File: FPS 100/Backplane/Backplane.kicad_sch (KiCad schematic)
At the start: 13 parts, among them J2 Conn_02x50_100pin

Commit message: 2026/1/3
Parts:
- added 4408_P3_J1, 4408_P3_J2, 4422_P1_J3, 4422_P1_J4, 4423_P2_J1, 4423_P2_J2, Spare1_J1, Spare1_J2: Conn_02x60_120pin, symbol User:Conn_02x60_120pin
- added 4421_PDP_IF_J1, 4421_PDP_IF_J2, 4429_FMT_J1, 4429_FMT_J2, Spare2_J2, Spare2_J3, Spare2_J4: Conn_02x50_100pin, symbol User:Conn_02x50_100pin
- renumbered J2 to Spare2_J1
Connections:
- net +5V: now also Spare2_J1.1, Spare2_J1.100, Spare2_J1.2, Spare2_J1.99, 4408_P3_J1.1, 4408_P3_J1.119, 4408_P3_J1.120, 4408_P3_J1.2, 4408_P3_J2.1, 4408_P3_J2.119, 4408_P3_J2.120, 4408_P3_J2.2, 4421_PDP_IF_J1.1, 4421_PDP_IF_J1.100, 4421_PDP_IF_J1.2, 4421_PDP_IF_J1.99, 4421_PDP_IF_J2.1, 4421_PDP_IF_J2.100, 4421_PDP_IF_J2.2, 4421_PDP_IF_J2.99, 4422_P1_J3.1, 4422_P1_J3.119, 4422_P1_J3.120, 4422_P1_J3.2, 4422_P1_J4.1, 4422_P1_J4.119, 4422_P1_J4.120, 4422_P1_J4.2, 4423_P2_J1.1, 4423_P2_J1.119, 4423_P2_J1.120, 4423_P2_J1.2, 4423_P2_J2.1, 4423_P2_J2.119, 4423_P2_J2.120, 4423_P2_J2.2, 4429_FMT_J1.1, 4429_FMT_J1.100, 4429_FMT_J1.2, 4429_FMT_J1.99, 4429_FMT_J2.1, 4429_FMT_J2.100, 4429_FMT_J2.2, 4429_FMT_J2.99, Spare1_J1.1, Spare1_J1.119, Spare1_J1.120, Spare1_J1.2, Spare1_J2.1, Spare1_J2.119, Spare1_J2.120, Spare1_J2.2, Spare2_J2.1, Spare2_J2.100, Spare2_J2.2, Spare2_J2.99, Spare2_J3.1, Spare2_J3.100, Spare2_J3.2, Spare2_J3.99, Spare2_J4.1, Spare2_J4.100, Spare2_J4.2, Spare2_J4.99
- net ABORT*: now also 4423_P2_J2.19
- net BPPENB*: now also 4423_P2_J2.57
- net BS2M1: now also 4423_P2_J2.45
- net BS2M2: now also 4423_P2_J2.46
- net DP2DP: now also 4423_P2_J1.112
- net DP2M1: now also 4423_P2_J2.50
- net DP2M2: now also 4423_P2_J2.52
- net DPEBS02*: now also 4423_P2_J1.79
- net DPEBS03*: now also 4423_P2_J1.80
- net DPEBS04*: now also 4423_P2_J1.99
- net DPEBS05*: now also 4423_P2_J1.100
- net DPEBS06*: now also 4423_P2_J1.101
- net DPEBS07*: now also 4423_P2_J1.102
- net DPEBS08*: now also 4423_P2_J2.5
- net DPEBS09*: now also 4423_P2_J2.6
- net DPEBS10*: now also 4423_P2_J2.7
- net DPEBS11*: now also 4423_P2_J2.8
- net DPMBS00*: now also 4423_P2_J2.27
- net DPMBS01*: now also 4423_P2_J2.28
- net DPMBS02*: now also 4423_P2_J2.29
- net DPMBS03*: now also 4423_P2_J2.30
- net DPMBS04*: now also 4423_P2_J2.33
- net DPMBS05*: now also 4423_P2_J2.34
- net DPMBS06*: now also 4423_P2_J2.35
- net DPMBS07*: now also 4423_P2_J2.36
- net DPMBS08*: now also 4423_P2_J2.41
- net DPMBS09*: now also 4423_P2_J2.42
- net DPMBS10*: now also 4423_P2_J2.43
- net DPMBS11*: now also 4423_P2_J2.44
- net DPMBS12*: now also 4423_P2_J2.69
- net DPMBS13*: now also 4423_P2_J2.70
- net DPMBS14*: now also 4423_P2_J2.71
- net DPMBS15*: now also 4423_P2_J2.72
- net DPMBS16*: now also 4423_P2_J2.77
- net DPMBS17*: now also 4423_P2_J2.78
- net DPMBS18*: now also 4423_P2_J2.79
- net DPMBS19*: now also 4423_P2_J2.80
- net DPMBS20*: now also 4423_P2_J2.95
- net DPMBS21*: now also 4423_P2_J2.96
- net DPMBS22*: now also 4423_P2_J2.97
- net DPMBS23*: now also 4423_P2_J2.98
- net DPMBS24*: now also 4423_P2_J2.109
- net DPMBS25*: now also 4423_P2_J2.110
- net DPMBS26*: now also 4423_P2_J2.111
- net DPMBS27*: now also 4423_P2_J2.112
- net FMUL*: now also 4423_P2_J2.61
- net GND: now also Spare2_J1.3, Spare2_J1.4, Spare2_J1.97, Spare2_J1.98, 4408_P3_J1.117, 4408_P3_J1.118, 4408_P3_J1.3, 4408_P3_J1.4, 4408_P3_J2.117, 4408_P3_J2.118, 4408_P3_J2.3, 4408_P3_J2.4, 4421_PDP_IF_J1.3, 4421_PDP_IF_J1.4, 4421_PDP_IF_J1.97, 4421_PDP_IF_J1.98, 4421_PDP_IF_J2.3, 4421_PDP_IF_J2.4, 4421_PDP_IF_J2.97, 4421_PDP_IF_J2.98, 4422_P1_J3.117, 4422_P1_J3.118, 4422_P1_J3.3, 4422_P1_J3.4, 4422_P1_J4.117, 4422_P1_J4.118, 4422_P1_J4.3, 4422_P1_J4.4, 4423_P2_J1.117, 4423_P2_J1.118, 4423_P2_J1.3, 4423_P2_J1.4, 4423_P2_J2.117, 4423_P2_J2.118, 4423_P2_J2.3, 4423_P2_J2.4, 4429_FMT_J1.3, 4429_FMT_J1.4, 4429_FMT_J1.97, 4429_FMT_J1.98, 4429_FMT_J2.3, 4429_FMT_J2.4, 4429_FMT_J2.97, 4429_FMT_J2.98, Spare1_J1.117, Spare1_J1.118, Spare1_J1.3, Spare1_J1.4, Spare1_J2.117, Spare1_J2.118, Spare1_J2.3, Spare1_J2.4, Spare2_J2.3, Spare2_J2.4, Spare2_J2.97, Spare2_J2.98, Spare2_J3.3, Spare2_J3.4, Spare2_J3.97, Spare2_J3.98, Spare2_J4.3, Spare2_J4.4, Spare2_J4.97, Spare2_J4.98
- net MACE*: now also 4423_P2_J2.102
- net MAINC*: now also 4423_P2_J2.55
- net MALD*: now also 4423_P2_J2.103
- net MD2DP: now also 4423_P2_J1.111
- net MD2M2: now also 4423_P2_J2.56
- net MDCR3*: now also 4423_P2_J2.101
- net MDWRT3: now also 4423_P2_J2.54
- net MIA*: now also 4423_P2_J2.105
- net MIB*: now also 4423_P2_J2.106
- net SAMEX: now also 4423_P2_J1.19
- net SAMEY: now also 4423_P2_J1.20
- net SP+DP00*: now also 4423_P2_J1.29
- net SP+DP01*: now also 4423_P2_J1.30
- net SP+DP02*: now also 4423_P2_J1.31
- net SP+DP03*: now also 4423_P2_J1.32
- net SP+DP04*: now also 4423_P2_J1.51
- net SP+DP05*: now also 4423_P2_J1.52
- net SP+DP06*: now also 4423_P2_J1.53
- net SP+DP07*: now also 4423_P2_J1.54
- net SP+DP08*: now also 4423_P2_J1.59
- net SP+DP09*: now also 4423_P2_J1.60
- net SP+DP10*: now also 4423_P2_J1.61
- net SP+DP11*: now also 4423_P2_J1.62
- net SP+DP12*: now also 4423_P2_J1.75
- net SP+DP13*: now also 4423_P2_J1.76
- net SP+DP14*: now also 4423_P2_J1.77
- net SP+DP15*: now also 4423_P2_J1.78
- net TM2DP: now also 4423_P2_J1.109
- net TM2M1: now also 4423_P2_J2.51
- net TMA00: now also 4423_P2_J1.25
- net TMA01: now also 4423_P2_J1.26
- net TMA02: now also 4423_P2_J1.27
- net TMA03: now also 4423_P2_J1.28
- net TMA04: now also 4423_P2_J1.47
- net TMA05: now also 4423_P2_J1.48
- net TMA06: now also 4423_P2_J1.49
- net TMA07: now also 4423_P2_J1.50
- net TMA08: now also 4423_P2_J1.55
- net TMA09: now also 4423_P2_J1.56
- net TMA10: now also 4423_P2_J1.57
- net TMA11: now also 4423_P2_J1.58
- net TMA12: now also 4423_P2_J1.71
- net TMA13: now also 4423_P2_J1.72
- net TMA14: now also 4423_P2_J1.73
- net TMA15: now also 4423_P2_J1.74
- net TMINH: now also 4423_P2_J1.38
- net TMNEG: now also 4423_P2_J1.36
- net TMREGE: now also 4423_P2_J2.113
- net WRTEXP: now also 4423_P2_J1.97
- net WRTHM: now also 4423_P2_J1.96
- net WRTLM: now also 4423_P2_J1.95
- net X01: now also 4423_P2_J1.9
- net X02: now also 4423_P2_J1.11
- net X03: now also 4423_P2_J1.13
- net X04: now also 4423_P2_J1.15
- net X05: now also 4423_P2_J1.17
- net XECLKE*: now also 4423_P2_J1.81
- net XHMCLKE*: now also 4423_P2_J1.82
- net XIA: now also 4423_P2_J1.84
- net XIB: now also 4423_P2_J1.89
- net XLMCLKE*: now also 4423_P2_J1.83
- net Y01: now also 4423_P2_J1.10
- net Y02: now also 4423_P2_J1.12
- net Y03: now also 4423_P2_J1.14
- net Y04: now also 4423_P2_J1.16
- net Y05: now also 4423_P2_J1.18
- net Y2DP: now also 4423_P2_J1.113
- net Y2M1: now also 4423_P2_J2.49
- net Y2M2: now also 4423_P2_J2.53
- net YECLKE*: now also 4423_P2_J1.86
- net YHMCLKE*: now also 4423_P2_J1.87
- net YIA: now also 4423_P2_J1.85
- net YIB: now also 4423_P2_J1.90
- net YLMCLKE*: now also 4423_P2_J1.88
- new net !CBCLK2: 4423_P2_J1.5
- new net !WRT*: 4423_P2_J1.6
- new net 376IN*: 4423_P2_J2.14
- new net 376LD*: 4423_P2_J2.26
- new net BMD2M2: 4423_P2_J2.48
- new net CBCLKE*: 4423_P2_J1.94
- new net DPA2PNL*: 4423_P2_J1.22
- new net DPALD*: 4423_P2_J1.21
- new net EX2PNL*: 4423_P2_J2.21
- new net EXIA: 4423_P2_J2.25
- new net EXIB: 4423_P2_J2.24
- new net FFTQ: 4423_P2_J1.35
- new net HD2DP: 4423_P2_J1.114
- new net IFFTQ: 4423_P2_J1.34
- new net INCCIN*: 4423_P2_J2.64
- new net MALD*A: 4423_P2_J2.65
- new net NEWINS1: 4423_P2_J2.81
- new net NEWINS2: 4423_P2_J2.82
- new net NEWINS3: 4423_P2_J2.83
- new net PLN00*: 4423_P2_J1.39
- new net PLN01*: 4423_P2_J1.40
- new net PLN02*: 4423_P2_J1.41
- new net PLN03*: 4423_P2_J1.42
- new net PLN04*: 4423_P2_J1.43
- new net PLN05*: 4423_P2_J1.44
- new net PLN06*: 4423_P2_J1.45
- new net PLN07*: 4423_P2_J1.46
- new net PLN08*: 4423_P2_J1.63
- new net PLN09*: 4423_P2_J1.64
- new net PLN10*: 4423_P2_J1.65
- new net PLN11*: 4423_P2_J1.66
- new net PLN12*: 4423_P2_J1.67
- new net PLN13*: 4423_P2_J1.68
- new net PLN14*: 4423_P2_J1.69
- new net PLN15*: 4423_P2_J1.70
- new net PNL2DP: 4423_P2_J1.92
- new net PNL2MA*: 4423_P2_J2.66
- new net PNL2TMA*: 4423_P2_J2.115
- new net PS1WRT: 4423_P2_J1.115
- new net PS24*A: 4423_P2_J1.103
- new net PS25*A: 4423_P2_J1.104
- new net PS26*A: 4423_P2_J1.105
- new net PS2WRT: 4423_P2_J1.116
- new net PS33*: 4423_P2_J2.9
- new net PS35*: 4423_P2_J2.10
- new net PS36*: 4423_P2_J2.11
- new net PS37*: 4423_P2_J2.12
- new net PS38*: 4423_P2_J2.13
- new net PS3WRT: 4423_P2_J2.58
- new net PS56*: 4423_P2_J2.87
- new net PS57*: 4423_P2_J2.89
- new net PS59*: 4423_P2_J2.90
- new net PS61*: 4423_P2_J2.92
- new net PS62*: 4423_P2_J2.93
- new net PS63*: 4423_P2_J2.94
- new net PSA04*: 4423_P2_J2.37
- new net PSA05*: 4423_P2_J2.38
- new net PSA06*: 4423_P2_J2.39
- new net PSA07*: 4423_P2_J2.40
- new net PSA08*: 4423_P2_J2.59
- new net PSA09*: 4423_P2_J2.60
- new net PSA10*: 4423_P2_J2.73
- new net PSA11*: 4423_P2_J2.74
- new net PSA12*: 4423_P2_J2.85
- new net PSA13*: 4423_P2_J2.86
- new net PSA14*: 4423_P2_J2.107
- new net PSA15*: 4423_P2_J2.108
- new net PSA2PNL: 4423_P2_J2.32
- new net PSAAD: 4423_P2_J2.16
- new net PSABD: 4423_P2_J2.17
- new net PSACD: 4423_P2_J2.18
- new net PSACLKE*: 4423_P2_J2.31
- new net PSH2DP: 4423_P2_J1.107
- new net PSL2DP: 4423_P2_J1.106
- new net PSZIP*: 4423_P2_J1.98
- new net RBUFQ: 4423_P2_J1.23
- new net SETATMA*: 4423_P2_J2.100
- new net SP2DP: 4423_P2_J1.110
- new net SPIN*: 4423_P2_J1.93
- new net SRADEC: 4423_P2_J2.22
- new net SRAINC: 4423_P2_J2.23
- new net SRAOVD: 4423_P2_J2.47
- new net SRSWE*: 4423_P2_J2.20
- new net TM2PNL: 4423_P2_J2.116
- new net TMA2PNL: 4423_P2_J1.37
- new net TMALD*A: 4423_P2_J2.114
- new net TSPIN: 4423_P2_J2.15
- new net USECB*: 4423_P2_J1.108
- new net WDPI: 4423_P2_J1.24
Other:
- note added: "FMT"
- note added: "P1 (4K)"
- note added: "P2 (4K)"
- note added: "P3"
- note added: "PDP-11 I/F"
- note added: "SPARE"
- moved on the sheet: 4401_FA_J1, 4401_FA_J2, 4402_DPL_J1, 4402_DPL_J2, 4402_DPR_J1, 4402_DPR_J2, 4424_MD_J1, 4424_MD_J2, 4425_TM_J1, 4425_TM_J2, 4426_FM_J1, 4426_FM_J2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

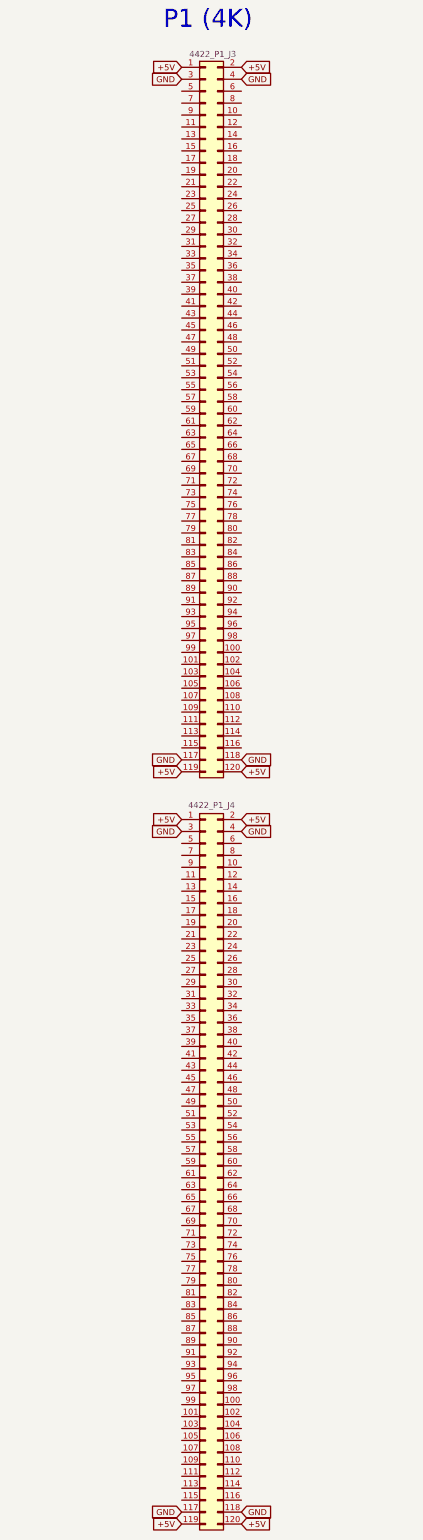
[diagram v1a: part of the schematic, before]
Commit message: 2026/1/3
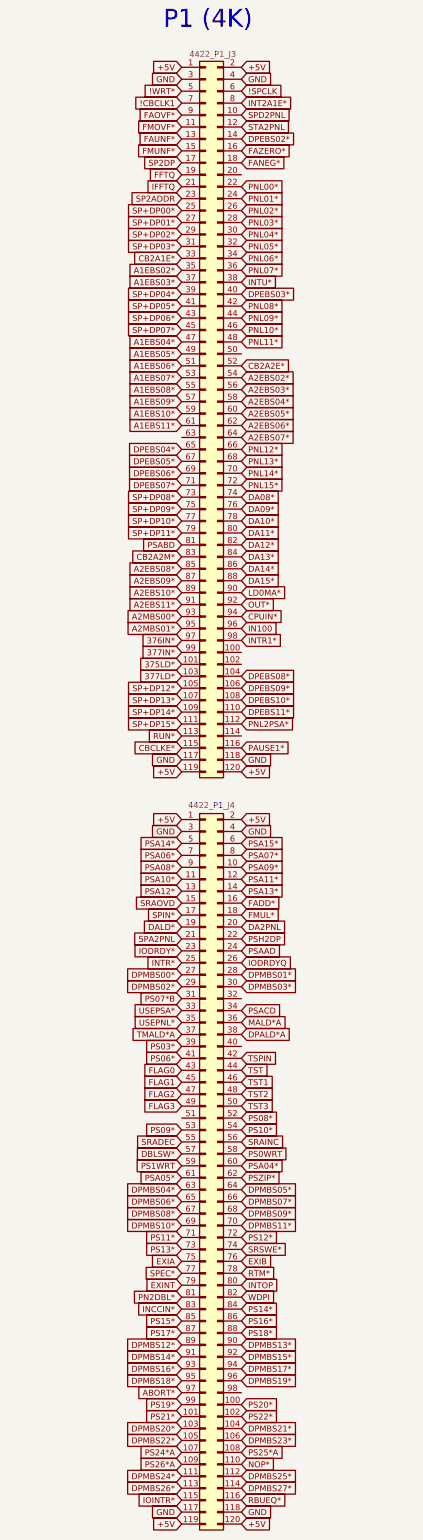
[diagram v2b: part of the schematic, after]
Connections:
- net !WRT*: now also 4422_P1_J3.5
- net 376IN*: now also 4422_P1_J3.97
- net A1EBS02*: now also 4422_P1_J3.35
- net A1EBS03*: now also 4422_P1_J3.37
- net A1EBS04*: now also 4422_P1_J3.47
- net A1EBS05*: now also 4422_P1_J3.49
- net A1EBS06*: now also 4422_P1_J3.51
- net A1EBS07*: now also 4422_P1_J3.53
- net A1EBS08*: now also 4422_P1_J3.55
- net A1EBS09*: now also 4422_P1_J3.57
- net A1EBS10*: now also 4422_P1_J3.59
- net A1EBS11*: now also 4422_P1_J3.61
- net A2EBS02*: now also 4422_P1_J3.54
- net A2EBS03*: now also 4422_P1_J3.56
- net A2EBS04*: now also 4422_P1_J3.58
- net A2EBS05*: now also 4422_P1_J3.60
- net A2EBS06*: now also 4422_P1_J3.62
- net A2EBS07*: now also 4422_P1_J3.64
- net A2EBS08*: now also 4422_P1_J3.85
- net A2EBS09*: now also 4422_P1_J3.87
- net A2EBS10*: now also 4422_P1_J3.89
- net A2EBS11*: now also 4422_P1_J3.91
- net A2MBS00*: now also 4422_P1_J3.93
- net A2MBS01*: now also 4422_P1_J3.95
- net ABORT*: now also 4422_P1_J4.97
- net CBCLKE*: now also 4422_P1_J3.115
- net DA08*: now also 4422_P1_J3.74
- net DA09*: now also 4422_P1_J3.76
- net DA10*: now also 4422_P1_J3.78
- net DA11*: now also 4422_P1_J3.80
- net DA12*: now also 4422_P1_J3.82
- net DA13*: now also 4422_P1_J3.84
- net DA14*: now also 4422_P1_J3.86
- net DA15*: now also 4422_P1_J3.88
- net DPEBS02*: now also 4422_P1_J3.14
- net DPEBS03*: now also 4422_P1_J3.40
- net DPEBS04*: now also 4422_P1_J3.65
- net DPEBS05*: now also 4422_P1_J3.67
- net DPEBS06*: now also 4422_P1_J3.69
- net DPEBS07*: now also 4422_P1_J3.71
- net DPEBS08*: now also 4422_P1_J3.104
- net DPEBS09*: now also 4422_P1_J3.106
- net DPEBS10*: now also 4422_P1_J3.108
- net DPEBS11*: now also 4422_P1_J3.110
- net DPMBS00*: now also 4422_P1_J4.27
- net DPMBS01*: now also 4422_P1_J4.28
- net DPMBS02*: now also 4422_P1_J4.29
- net DPMBS03*: now also 4422_P1_J4.30
- net DPMBS04*: now also 4422_P1_J4.63
- net DPMBS05*: now also 4422_P1_J4.64
- net DPMBS06*: now also 4422_P1_J4.65
- net DPMBS07*: now also 4422_P1_J4.66
- net DPMBS08*: now also 4422_P1_J4.67
- net DPMBS09*: now also 4422_P1_J4.68
- net DPMBS10*: now also 4422_P1_J4.69
- net DPMBS11*: now also 4422_P1_J4.70
- net DPMBS12*: now also 4422_P1_J4.89
- net DPMBS13*: now also 4422_P1_J4.90
- net DPMBS14*: now also 4422_P1_J4.91
- net DPMBS15*: now also 4422_P1_J4.92
- net DPMBS16*: now also 4422_P1_J4.93
- net DPMBS17*: now also 4422_P1_J4.94
- net DPMBS18*: now also 4422_P1_J4.95
- net DPMBS19*: now also 4422_P1_J4.96
- net DPMBS20*: now also 4422_P1_J4.103
- net DPMBS21*: now also 4422_P1_J4.104
- net DPMBS22*: now also 4422_P1_J4.105
- net DPMBS23*: now also 4422_P1_J4.106
- net DPMBS24*: now also 4422_P1_J4.111
- net DPMBS25*: now also 4422_P1_J4.112
- net DPMBS26*: now also 4422_P1_J4.113
- net DPMBS27*: now also 4422_P1_J4.114
- net EXIA: now also 4422_P1_J4.75
- net EXIB: now also 4422_P1_J4.76
- net FADD*: now also 4422_P1_J4.16
- net FANEG*: now also 4422_P1_J3.18
- net FFTQ: now also 4422_P1_J3.19
- net FMOVF*: now also 4422_P1_J3.11
- net FMUL*: now also 4422_P1_J4.18
- net FMUNF*: now also 4422_P1_J3.15
- net IFFTQ: now also 4422_P1_J3.21
- net INCCIN*: now also 4422_P1_J4.83
- net MALD*A: now also 4422_P1_J4.36
- net OUT*: now also 4422_P1_J3.92
- net PNL00*: now also 4422_P1_J3.22
- net PNL01*: now also 4422_P1_J3.24
- net PNL02*: now also 4422_P1_J3.26
- net PNL03*: now also 4422_P1_J3.28
- net PNL04*: now also 4422_P1_J3.30
- net PNL05*: now also 4422_P1_J3.32
- net PNL06*: now also 4422_P1_J3.34
- net PNL07*: now also 4422_P1_J3.36
- net PNL08*: now also 4422_P1_J3.42
- net PNL09*: now also 4422_P1_J3.44
- net PNL10*: now also 4422_P1_J3.46
- net PNL11*: now also 4422_P1_J3.48
- net PNL12*: now also 4422_P1_J3.66
- net PNL13*: now also 4422_P1_J3.68
- net PNL14*: now also 4422_P1_J3.70
- net PNL15*: now also 4422_P1_J3.72
- net PS1WRT: now also 4422_P1_J4.59
- net PS24*A: now also 4422_P1_J4.107
- net PS25*A: now also 4422_P1_J4.108
- net PS26*A: now also 4422_P1_J4.109
- net PSA04*: now also 4422_P1_J4.60
- net PSA05*: now also 4422_P1_J4.61
- net PSA06*: now also 4422_P1_J4.7
- net PSA07*: now also 4422_P1_J4.8
- net PSA08*: now also 4422_P1_J4.9
- net PSA09*: now also 4422_P1_J4.10
- net PSA10*: now also 4422_P1_J4.11
- net PSA11*: now also 4422_P1_J4.12
- net PSA12*: now also 4422_P1_J4.13
- net PSA13*: now also 4422_P1_J4.14
- net PSA14*: now also 4422_P1_J4.5
- net PSA15*: now also 4422_P1_J4.6
- net PSAAD: now also 4422_P1_J4.24
- net PSABD: now also 4422_P1_J3.81
- net PSACD: now also 4422_P1_J4.34
- net PSH2DP: now also 4422_P1_J4.22
- net PSZIP*: now also 4422_P1_J4.62
- net SP+DP00*: now also 4422_P1_J3.25
- net SP+DP01*: now also 4422_P1_J3.27
- net SP+DP02*: now also 4422_P1_J3.29
- net SP+DP03*: now also 4422_P1_J3.31
- net SP+DP04*: now also 4422_P1_J3.39
- net SP+DP05*: now also 4422_P1_J3.41
- net SP+DP06*: now also 4422_P1_J3.43
- net SP+DP07*: now also 4422_P1_J3.45
- net SP+DP08*: now also 4422_P1_J3.73
- net SP+DP09*: now also 4422_P1_J3.75
- net SP+DP10*: now also 4422_P1_J3.77
- net SP+DP11*: now also 4422_P1_J3.79
- net SP+DP12*: now also 4422_P1_J3.105
- net SP+DP13*: now also 4422_P1_J3.107
- net SP+DP14*: now also 4422_P1_J3.109
- net SP+DP15*: now also 4422_P1_J3.111
- net SP2DP: now also 4422_P1_J3.17
- net SPIN*: now also 4422_P1_J4.17
- net SRADEC: now also 4422_P1_J4.55
- net SRAINC: now also 4422_P1_J4.56
- net SRAOVD: now also 4422_P1_J4.15
- net SRSWE*: now also 4422_P1_J4.74
- net TMALD*A: now also 4422_P1_J4.37
- net TSPIN: now also 4422_P1_J4.42
- net WDPI: now also 4422_P1_J4.82
- net SPD2PNL: now reaches 4422_P1_J3.10
- net 375LD*: now reaches 4422_P1_J3.101
- net 377LD*: now reaches 4422_P1_J3.103
- net PNL2PSA*: now reaches 4422_P1_J3.112
- net RUN*: now reaches 4422_P1_J3.113
- net PAUSE1*: now reaches 4422_P1_J3.116
- net STA2PNL: now reaches 4422_P1_J3.12
- net FAUNF*: now reaches 4422_P1_J3.13
- net FAZERO*: now reaches 4422_P1_J3.16
- net SP2ADDR: now reaches 4422_P1_J3.23
- net CB2A1E*: now reaches 4422_P1_J3.33
- net INTU*: now reaches 4422_P1_J3.38
- net CB2A2E*: now reaches 4422_P1_J3.52
- net !SPCLK: now reaches 4422_P1_J3.6
- net !CBCLK1: now reaches 4422_P1_J3.7
- net INT2A1E*: now reaches 4422_P1_J3.8
- net CB2A2M*: now reaches 4422_P1_J3.83
- net FAOVF*: now reaches 4422_P1_J3.9
- net LD0MA*: now reaches 4422_P1_J3.90
- net CPUIN*: now reaches 4422_P1_J3.94
- net IN100: now reaches 4422_P1_J3.96
- net INTR1*: now reaches 4422_P1_J3.98
- net 377IN*: now reaches 4422_P1_J3.99
- net PS20*: now reaches 4422_P1_J4.100
- net PS21*: now reaches 4422_P1_J4.101
- net PS22*: now reaches 4422_P1_J4.102
- net NOP*: now reaches 4422_P1_J4.110
- net IOINTR*: now reaches 4422_P1_J4.115
- net RBUEQ*: now reaches 4422_P1_J4.116
- net DALD*: now reaches 4422_P1_J4.19
- net DA2PNL: now reaches 4422_P1_J4.20
- net SPA2PNL: now reaches 4422_P1_J4.21
- net IODRDY*: now reaches 4422_P1_J4.23
- net INTR*: now reaches 4422_P1_J4.25
- net IODRDYQ: now reaches 4422_P1_J4.26
- net PS07*B: now reaches 4422_P1_J4.31
- net USEPSA*: now reaches 4422_P1_J4.33
- net USEPNL*: now reaches 4422_P1_J4.35
- net DPALD*A: now reaches 4422_P1_J4.38
- net PS03*: now reaches 4422_P1_J4.39
- net PS06*: now reaches 4422_P1_J4.41
- net FLAG0: now reaches 4422_P1_J4.43
- net TST: now reaches 4422_P1_J4.44
- net FLAG1: now reaches 4422_P1_J4.45
- net TST1: now reaches 4422_P1_J4.46
- net FLAG2: now reaches 4422_P1_J4.47
- net TST2: now reaches 4422_P1_J4.48
- net FLAG3: now reaches 4422_P1_J4.49
- net TST3: now reaches 4422_P1_J4.50
- net PS08*: now reaches 4422_P1_J4.52
- net PS09*: now reaches 4422_P1_J4.53
- net PS10*: now reaches 4422_P1_J4.54
- net DBLSW*: now reaches 4422_P1_J4.57
- net PS0WRT: now reaches 4422_P1_J4.58
- net PS11*: now reaches 4422_P1_J4.71
- net PS12*: now reaches 4422_P1_J4.72
- net PS13*: now reaches 4422_P1_J4.73
- net SPEC*: now reaches 4422_P1_J4.77
- net RTM*: now reaches 4422_P1_J4.78
- net EXINT: now reaches 4422_P1_J4.79
- net INTOP: now reaches 4422_P1_J4.80
- net PN2DBL*: now reaches 4422_P1_J4.81
- net PS14*: now reaches 4422_P1_J4.84
- net PS15*: now reaches 4422_P1_J4.85
- net PS16*: now reaches 4422_P1_J4.86
- net PS17*: now reaches 4422_P1_J4.87
- net PS18*: now reaches 4422_P1_J4.88
- net PS19*: now reaches 4422_P1_J4.99
